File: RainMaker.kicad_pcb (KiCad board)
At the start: 2 copper layers, 130 x 72 mm, 78 parts, among them IC1 ESP32-WROOM-32D, J1 Screw Terminal - 2P, Q1 IRLR8726TRPBF, Q10 IRLR8726TRPBF, Q11 IRLR8726TRPBF, Q12 IRLR8726TRPBF, Q2 IRLR8726TRPBF, Q3 IRLR8726TRPBF, Q4 IRLR8726TRPBF, Q5 IRLR8726TRPBF, Q6 IRLR8726TRPBF, Q7 IRLR8726TRPBF, Q8 IRLR8726TRPBF, Q9 IRLR8726TRPBF, SW1 UK-B0206-G5-250-JZ, U1 TPS54202DDC

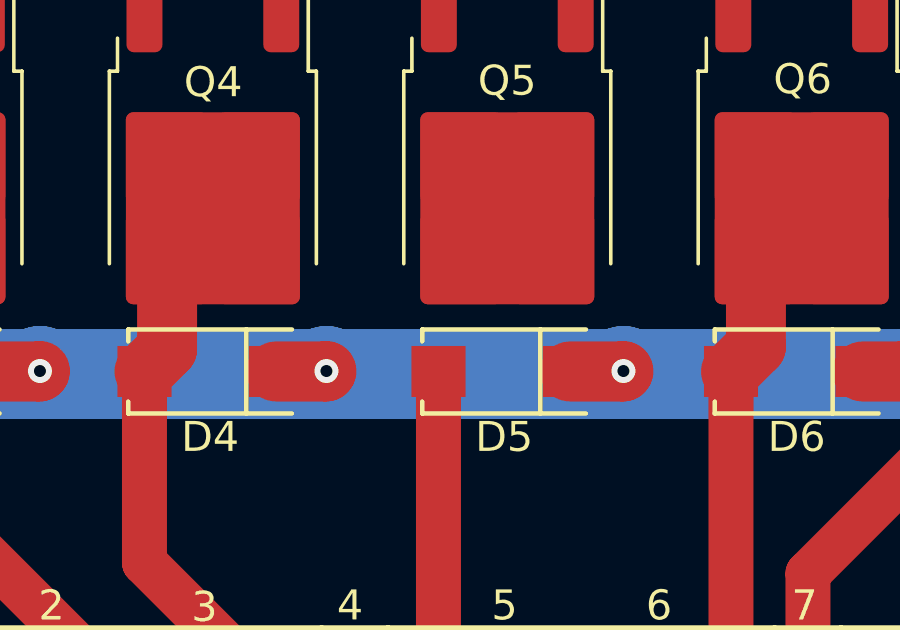
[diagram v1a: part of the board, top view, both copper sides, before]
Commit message: fix unconnected
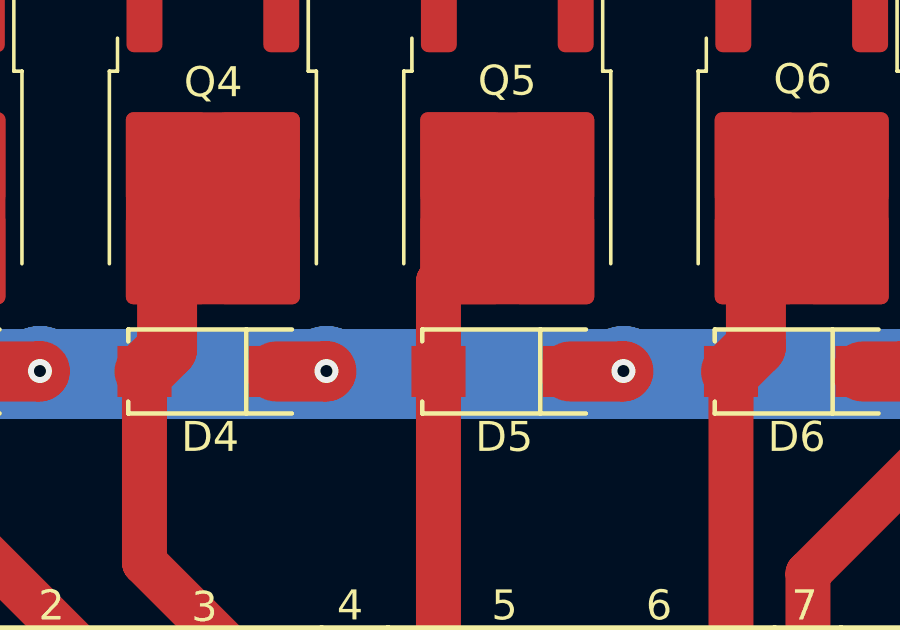
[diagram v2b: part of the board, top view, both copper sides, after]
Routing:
- net /Z_5_OUT: track 14.4 -> 18.5 mm
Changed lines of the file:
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@@
   (segment (start 87.485 102.665) (end 87.485 109.035) (width 1.5) (layer "F.Cu") (net 8))
   (segment (start 87.485 109.035) (end 94.6 116.15) (width 1.5) (layer "F.Cu") (net 8))
+  (segment (start 97.285 102.665) (end 97.285 99.668676) (width 1.5) (layer "F.Cu") (net 9))
+  (segment (start 97.285 99.668676) (end 98.053676 98.9) (width 1.5) (layer "F.Cu") (net 9))
   (segment (start 97.285 102.665) (end 97.285 113.835) (width 1.5) (layer "F.Cu") (net 9))
   (segment (start 97.285 113.835) (end 99.6 116.15) (width 1.5) (layer "F.Cu") (net 9))
